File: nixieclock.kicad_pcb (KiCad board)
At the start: 11 copper layers, 146.5 x 85 mm, 50 parts, among them Q1 MMBTA42, Q2 FDS2672CT, Q3 SS8050, U1 UCC3803, U2 K155NA1, U3 PicoW, U4 K155NA1, U5 K155NA1, U6 K155NA1, U7 K155NA1, U8 K155NA1

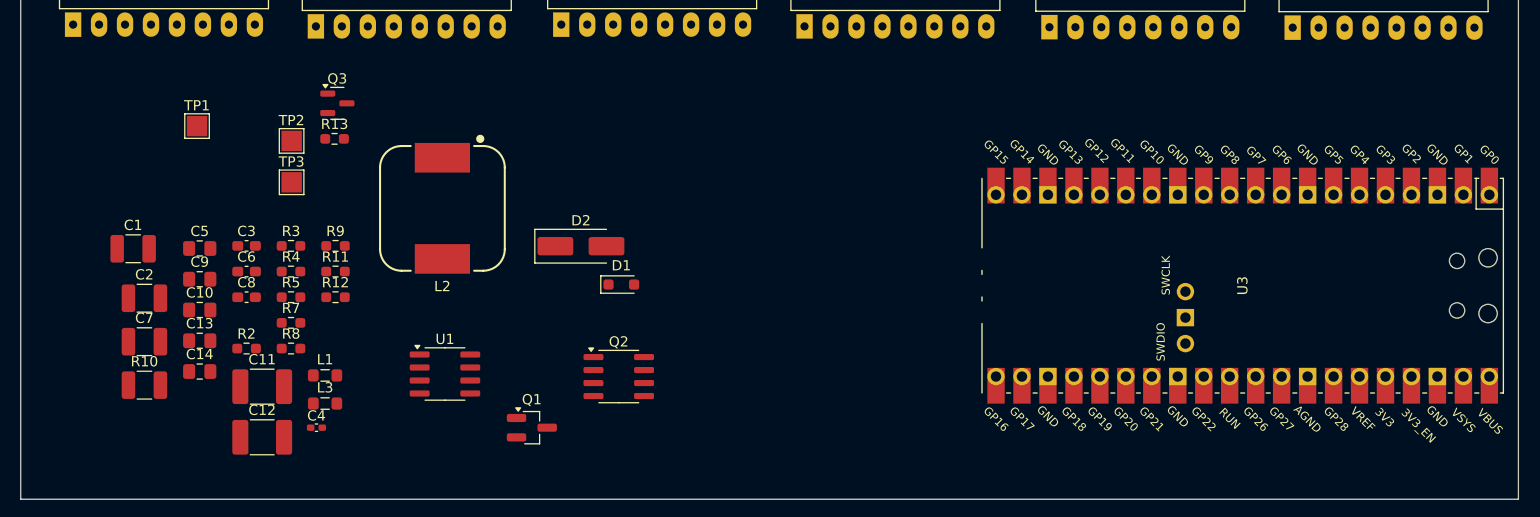
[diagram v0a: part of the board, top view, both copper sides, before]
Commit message: layout
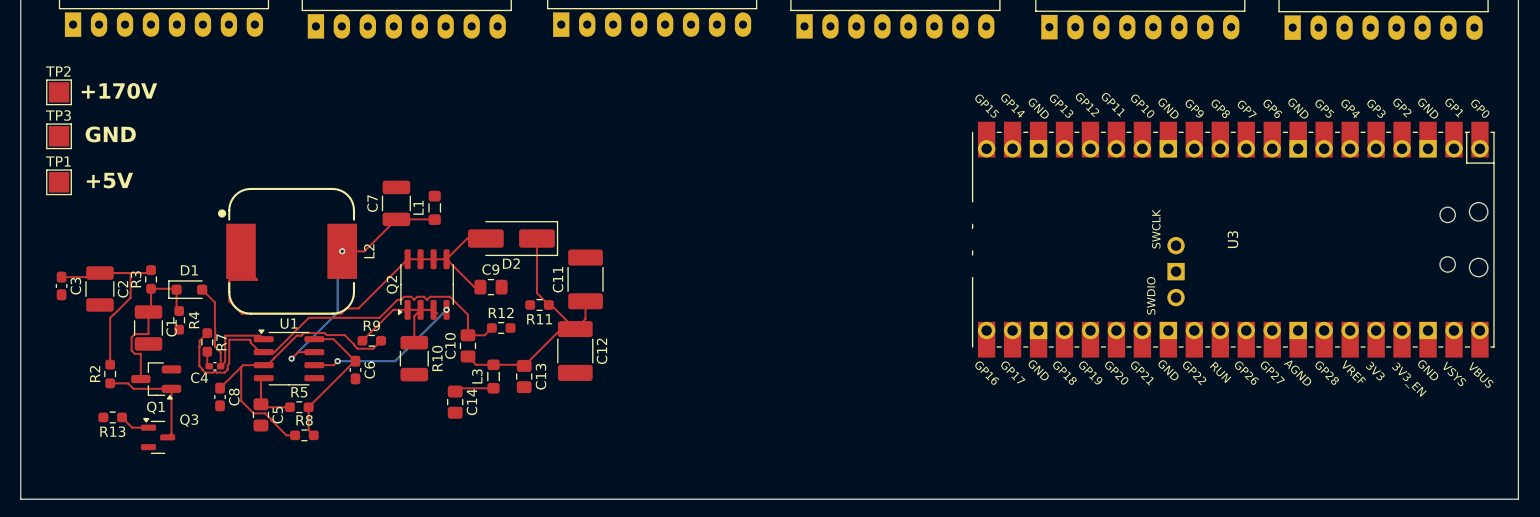
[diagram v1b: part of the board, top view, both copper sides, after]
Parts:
- moved D1 42.3 mm to (133.0, 90.0)
- moved Q3 37.1 mm to (129.9, 104.5)
- moved Q1 37.1 mm to (129.8, 98.8), turned to 180 degrees
- moved R13 34.8 mm to (125.5, 102.5), turned to 180 degrees
- moved C11 33.3 mm to (171.8, 89.0), turned to 90 degrees
- moved C13 31.9 mm to (165.8, 98.5), turned to -90 degrees
- moved C12 31.8 mm to (170.8, 96.0), turned to -90 degrees
- moved C9 28.5 mm to (162.5, 89.8)
- moved C7 28.1 mm to (153.2, 81.6), turned to 90 degrees
- moved R10 26.5 mm to (155.0, 96.8), turned to -90 degrees
- moved C10 26.5 mm to (160.2, 95.5), turned to 90 degrees
- moved C14 25.2 mm to (159.0, 101.0), turned to -90 degrees
- moved TP2 23.2 mm to (120.2, 70.7)
- moved TP3 23.2 mm to (120.2, 75.0)
- moved Q2 20.8 mm to (156.2, 89.5), turned to 90 degrees
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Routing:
- net Net-(U1-FB): track 0.00 -> 41.9 mm
- net Net-(D2-A): track 0.00 -> 41.3 mm
- net Net-(U1-Isense): track 0.00 -> 29.0 mm
- net Net-(D2-K): track 0.00 -> 26.1 mm
- net Net-(U1-Vcc): track 0.00 -> 26.0 mm, vias 0 -> 2
- net +5V: track 0.00 -> 18.9 mm
- net Net-(D1-K): track 0.00 -> 15.9 mm
- net Net-(D1-A): track 0.00 -> 15.4 mm
- net Net-(Q2-G): track 0.00 -> 15.2 mm, vias 0 -> 2
- net Net-(U1-Vref): track 0.00 -> 14.3 mm
- net Net-(Q2-S-Pad1): track 0.00 -> 12.2 mm
- net Net-(Q1-B): track 0.00 -> 11.1 mm
- net Net-(U1-R/C): track 0.00 -> 5.63 mm
- net +170V: track 0.00 -> 3.88 mm
- net Net-(Q3-B): track 0.00 -> 3.00 mm
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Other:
- board text added: "+170V"
- board text added: "+5V"
- board text added: "GND"

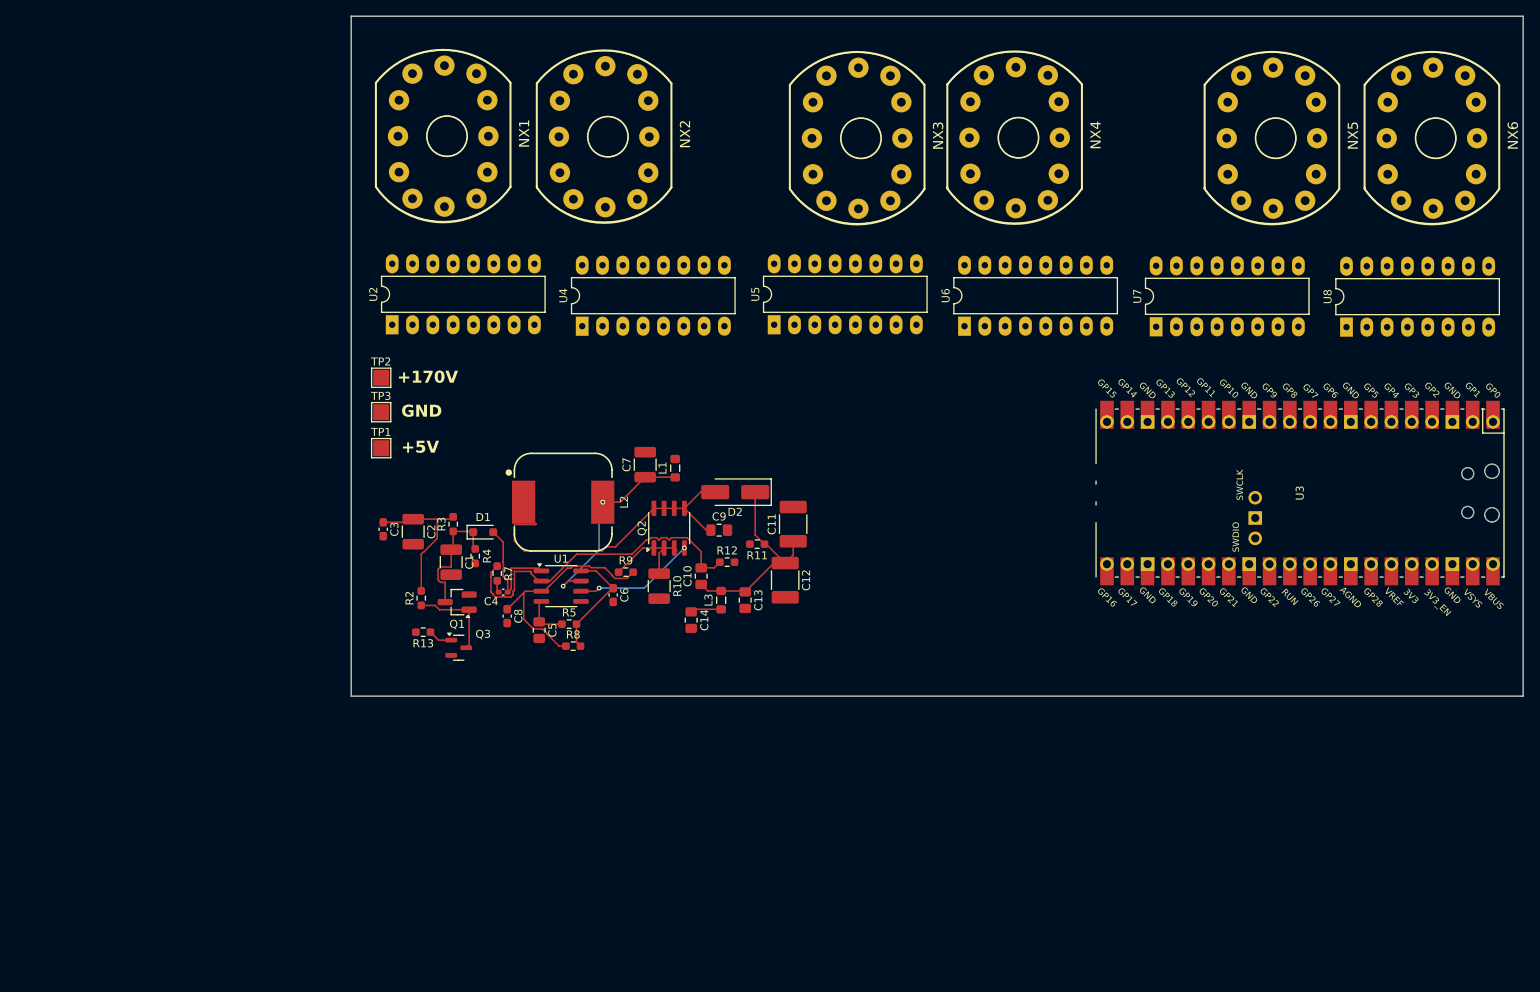
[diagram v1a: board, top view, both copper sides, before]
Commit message: mostly done i guess?
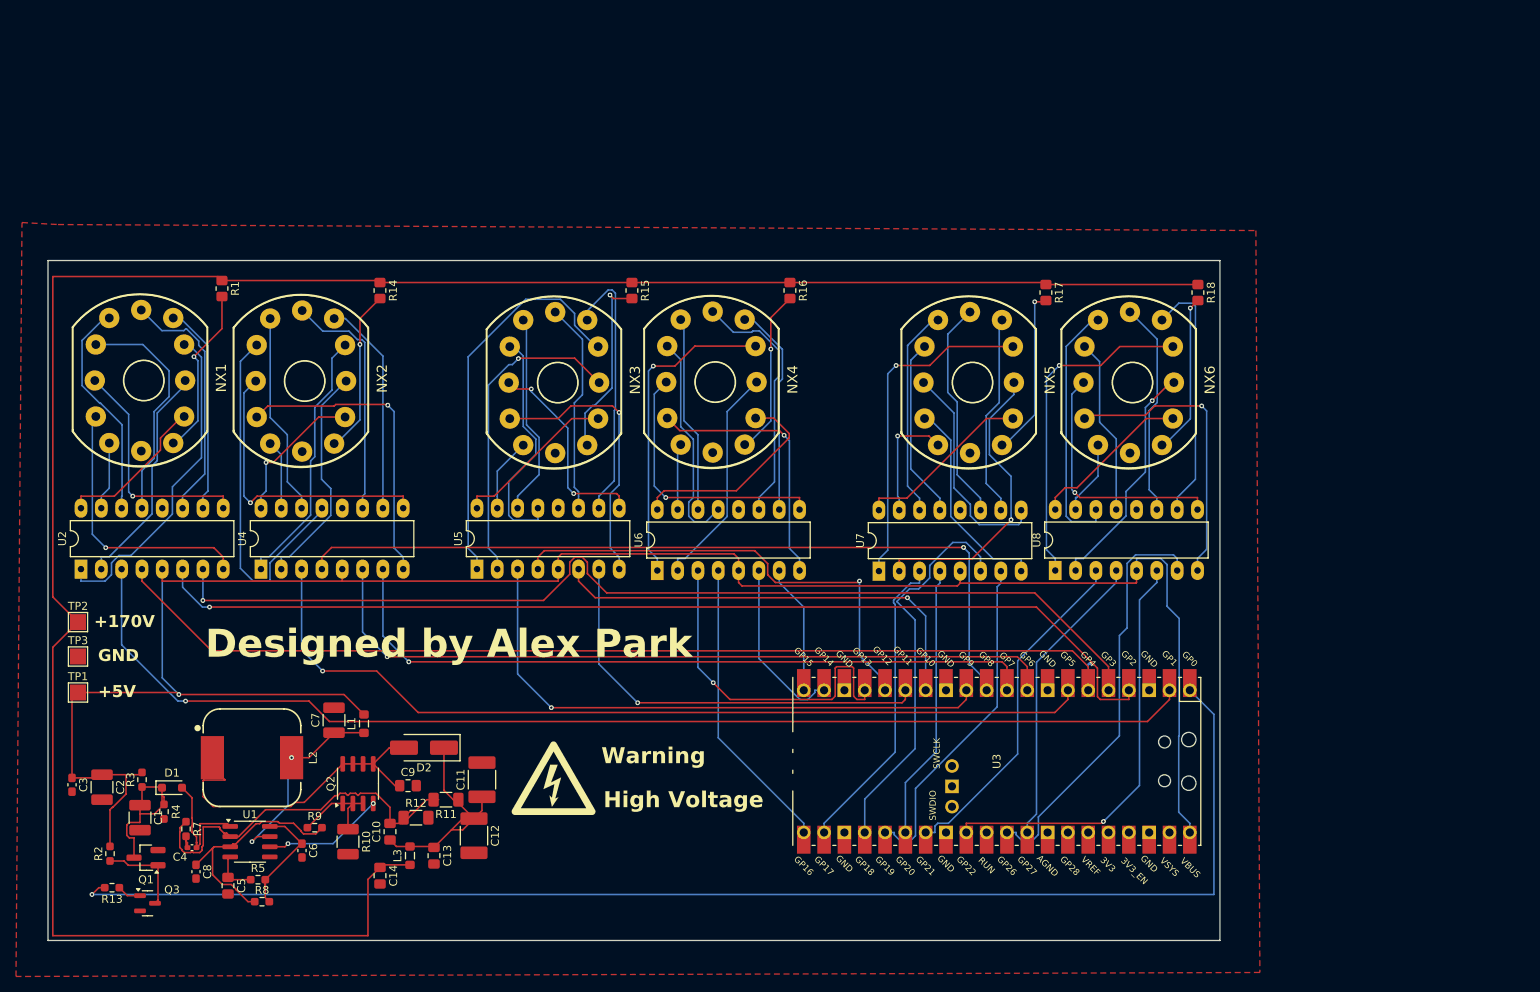
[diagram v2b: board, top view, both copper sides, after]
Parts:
- added R1: 10.5k, Resistor_SMD:R_0805_2012Metric_Pad1.20x1.40mm_HandSolder, F.Cu at (100.3, 59.5)
- added R14: 10.5k, Resistor_SMD:R_0805_2012Metric_Pad1.20x1.40mm_HandSolder, F.Cu at (120.1, 59.8)
- added R15: 10.5k, Resistor_SMD:R_0805_2012Metric_Pad1.20x1.40mm_HandSolder, F.Cu at (151.6, 59.8)
- added R16: 10.5k, Resistor_SMD:R_0805_2012Metric_Pad1.20x1.40mm_HandSolder, F.Cu at (171.3, 59.8)
- added R17: 10.5k, Resistor_SMD:R_0805_2012Metric_Pad1.20x1.40mm_HandSolder, F.Cu at (203.3, 60.0)
- added R18: 10.5k, Resistor_SMD:R_0805_2012Metric_Pad1.20x1.40mm_HandSolder, F.Cu at (222.3, 60.0)
- R11, R12: footprint Resistor_SMD:R_0603_1608Metric_Pad0.98x0.95mm_HandSolder -> Resistor_SMD:R_1206_3216Metric_Pad1.30x1.75mm_HandSolder
- moved U3 50.6 mm to (197.2, 118.7)
- moved U4 50.3 mm to (105.2, 94.6)
- moved C1 50.3 mm to (90.1, 125.7)
- moved C10 50.3 mm to (121.3, 127.4)
- moved C2 50.3 mm to (85.3, 121.9)
- moved C3 50.3 mm to (81.6, 121.6)
- moved C6 50.3 mm to (110.3, 129.8)
- moved C7 50.3 mm to (114.3, 113.5)
- moved C9 50.3 mm to (123.6, 121.7)
- moved D1 50.3 mm to (94.1, 121.9)
- moved D2 50.3 mm to (125.6, 116.9)
- moved L1 50.3 mm to (118.1, 113.9)
- moved L2 50.3 mm to (104.1, 118.2)
- moved Q2 50.3 mm to (117.3, 121.4)
- moved Q3 50.3 mm to (91.0, 136.4)
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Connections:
- NX1 pad A: unconnected-(NX1-PadA) -> Net-(NX1-PadA)
- NX2 pad A: unconnected-(NX2-PadA) -> Net-(NX2-PadA)
- NX3 pad A: unconnected-(NX3-PadA) -> Net-(NX3-PadA)
- NX4 pad A: unconnected-(NX4-PadA) -> Net-(NX4-PadA)
- NX5 pad A: unconnected-(NX5-PadA) -> Net-(NX5-PadA)
- NX6 pad A: unconnected-(NX6-PadA) -> Net-(NX6-PadA)
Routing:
- net +170V: track 3.88 -> 281.0 mm
- net +5V: track 18.9 -> 258.2 mm, vias 0 -> 1
- net GPIO0: track 0.00 -> 169.0 mm, vias 0 -> 1
- net GPIO1: track 0.00 -> 146.7 mm, vias 0 -> 1
- net GPIO4: track 0.00 -> 131.1 mm
- net GPIO3: track 0.00 -> 129.7 mm, vias 0 -> 1
- net GPIO2: track 0.00 -> 129.6 mm, vias 0 -> 1
- net GPIO5: track 0.00 -> 111.0 mm, vias 0 -> 1
- net GPIO8: track 0.00 -> 101.3 mm, vias 0 -> 1
- net GPIO6: track 0.00 -> 95.7 mm, vias 0 -> 1
- net GPIO7: track 0.00 -> 90.9 mm, vias 0 -> 1
- net GPIO9: track 0.00 -> 72.5 mm, vias 0 -> 1
- net GPIO12: track 0.00 -> 59.6 mm, vias 0 -> 1
- net GPIO10: track 0.00 -> 56.0 mm, vias 0 -> 1
- net GPIO11: track 0.00 -> 53.5 mm, vias 0 -> 1
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- added copper zone on F.Cu, net GND
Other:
- board text added: "Designed by Alex Park"
- board text added: "High Voltage"
- board text added: "Warning"
